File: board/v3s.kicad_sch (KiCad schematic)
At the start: 1 part, among them J1 Conn_01x02

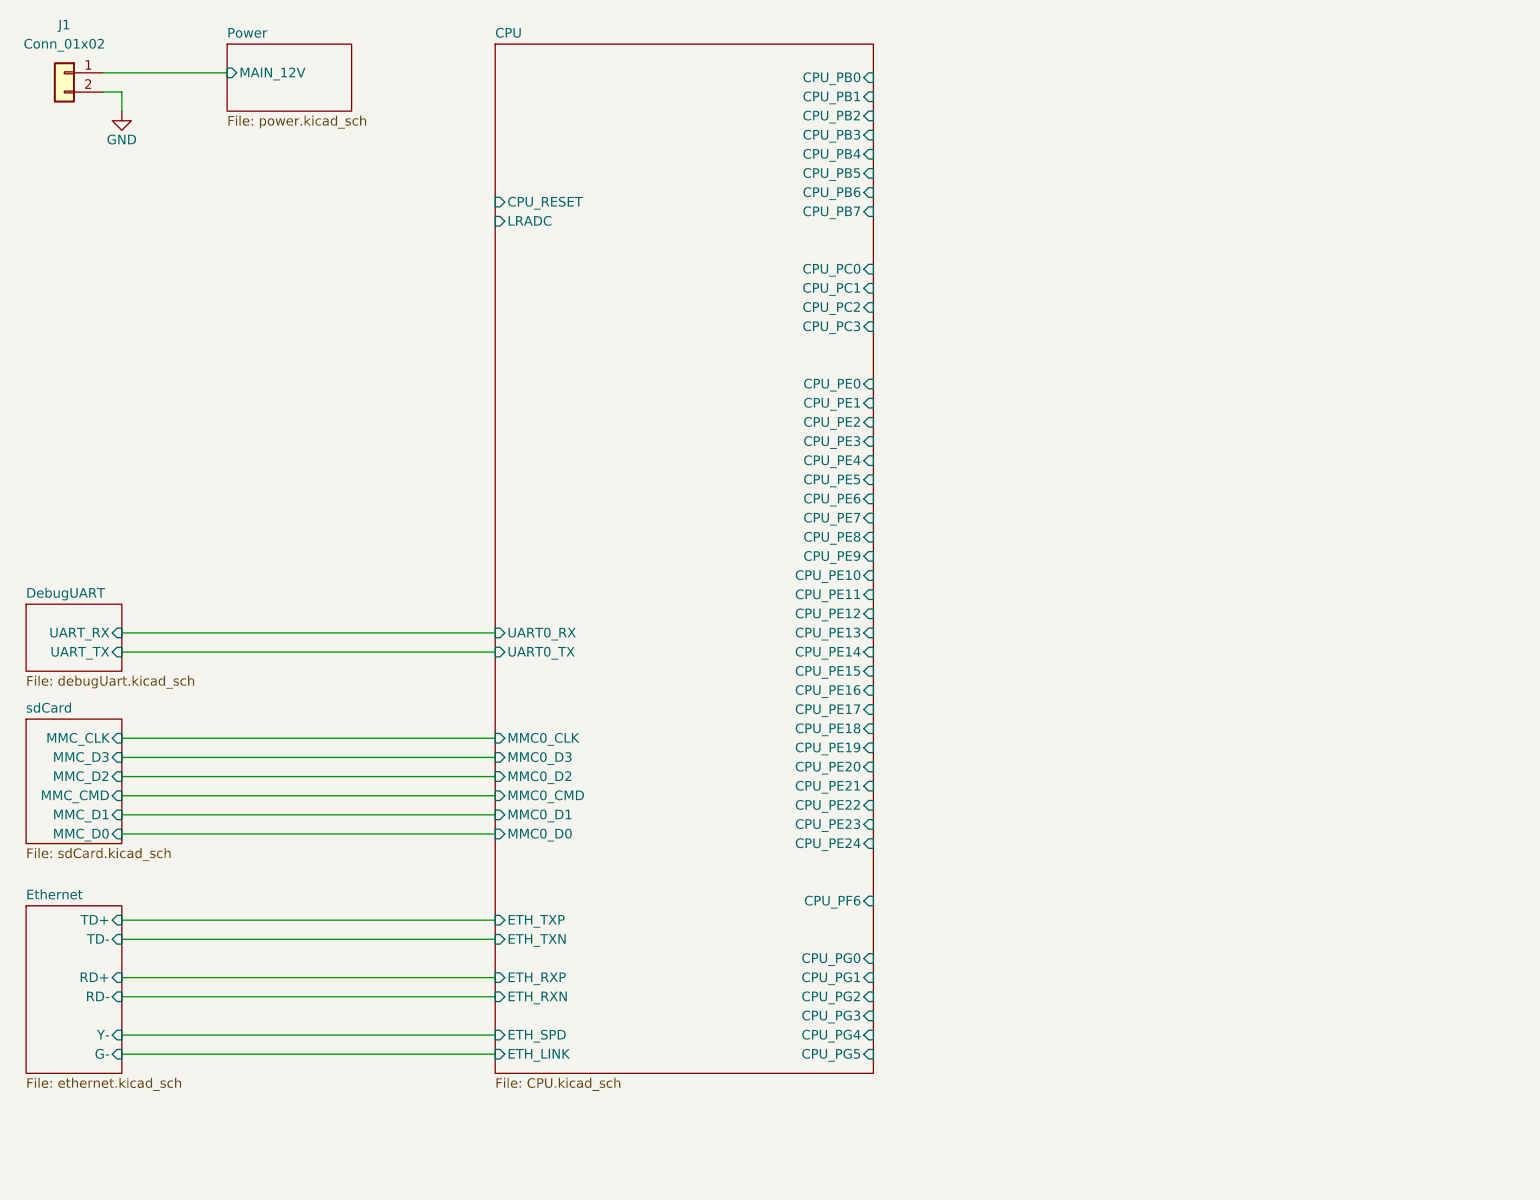
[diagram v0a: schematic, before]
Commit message: pcb layout
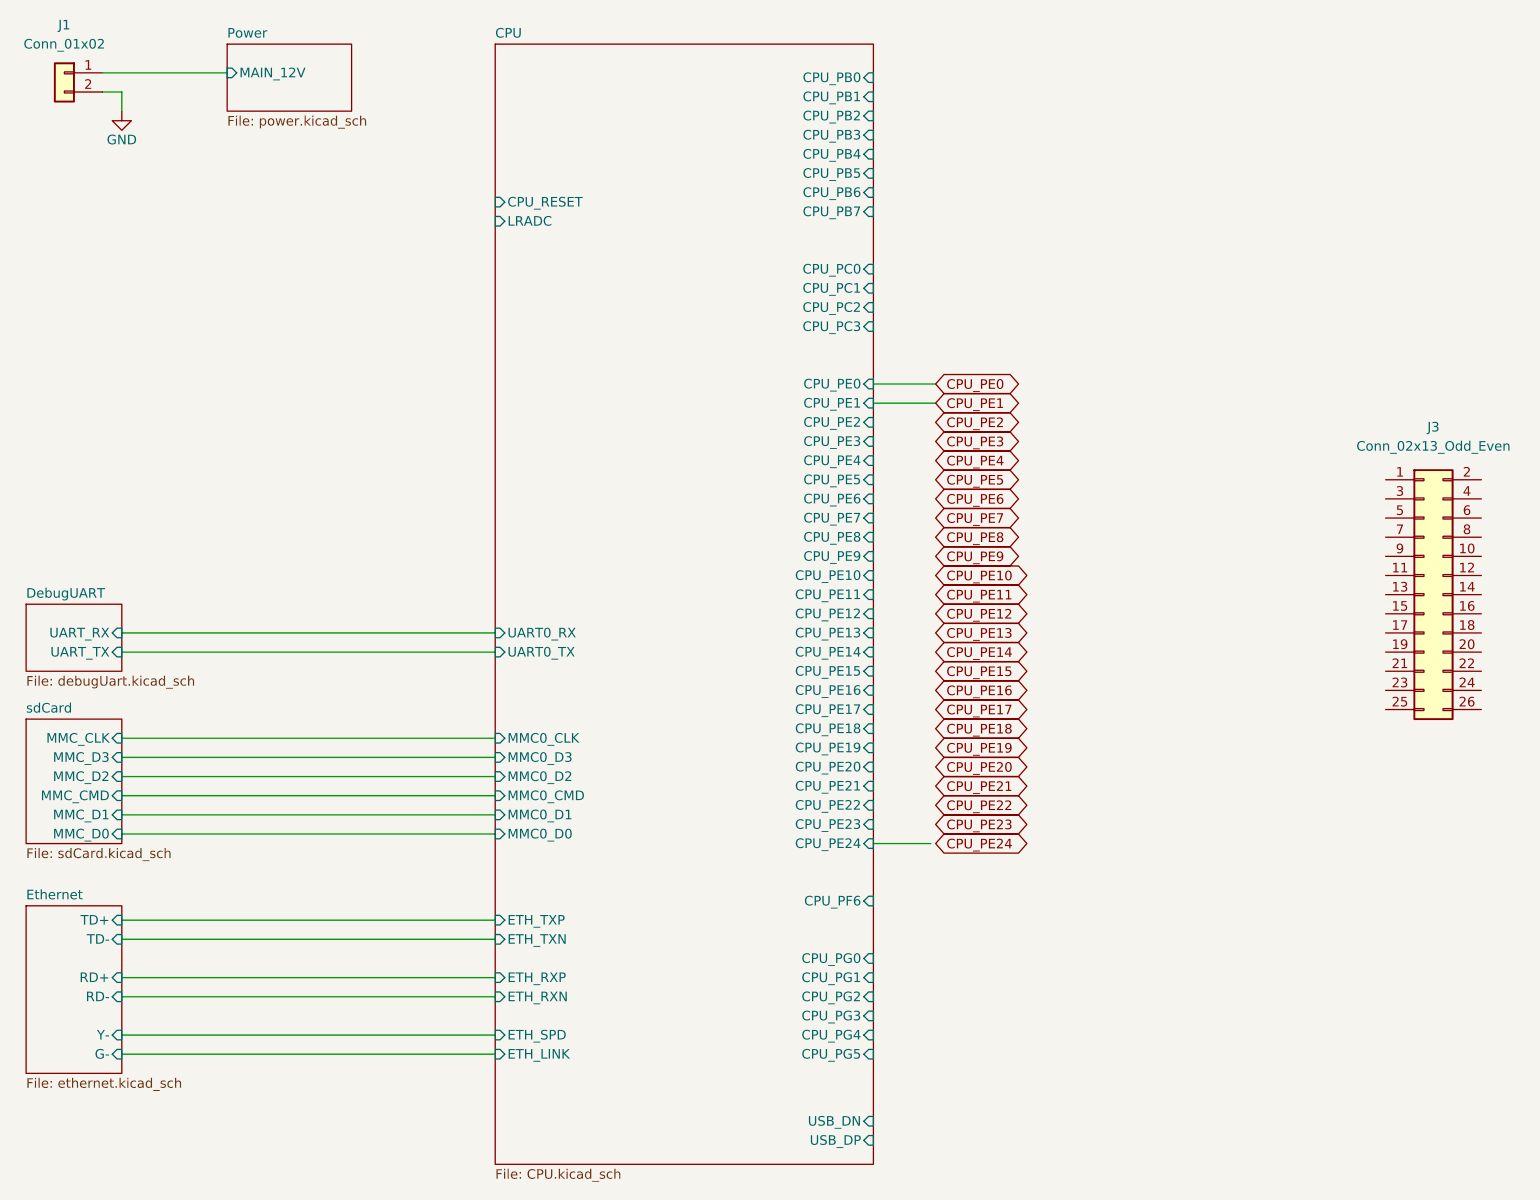
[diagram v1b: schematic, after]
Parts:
- added J3: Conn_02x13_Odd_Even, Connector_PinHeader_2.54mm:PinHeader_2x13_P2.54mm_Vertical, symbol Connector_Generic:Conn_02x13_Odd_Even
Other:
- sheet CPU ports: added USB_DN, USB_DP; removed none
